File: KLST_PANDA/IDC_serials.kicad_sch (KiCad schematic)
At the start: 0 parts

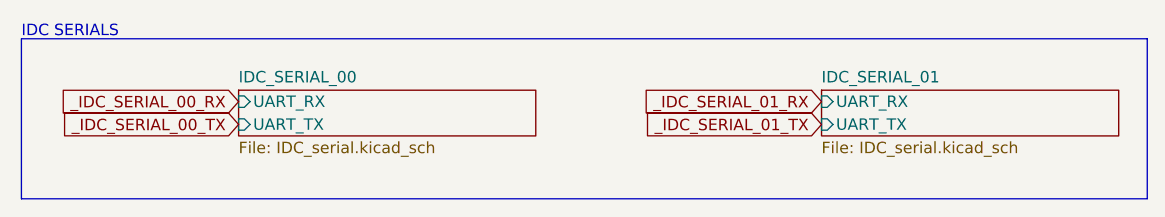
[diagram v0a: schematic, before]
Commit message: continued routing
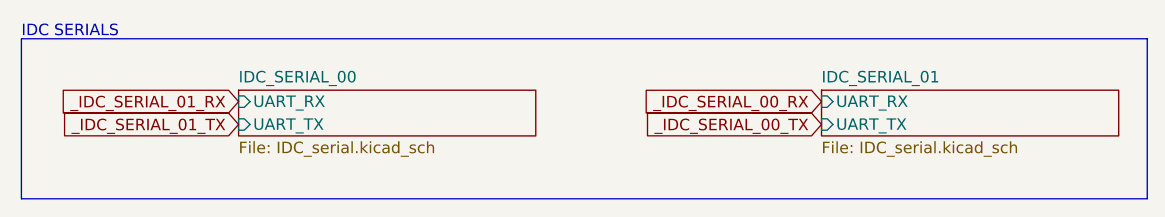
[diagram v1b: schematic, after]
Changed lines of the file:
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@@
     (effects (font (size 1.27 1.27)) (justify left bottom))
   )
-  (global_label "_IDC_SERIAL_00_TX" (shape input) (at 39.37 24.765 180) (fields_autoplaced)
+  (global_label "_IDC_SERIAL_00_TX" (shape input) (at 104.14 24.765 180) (fields_autoplaced)
+    (effects (font (size 1.27 1.27)) (justify right))
+    (property "Intersheetrefs" "${INTERSHEET_REFS}" (at 83.2729 24.765 0)
+      (effects (font (size 1.27 1.27)) (justify right) hide)
+    )
+  )
+  (global_label "_IDC_SERIAL_01_TX" (shape input) (at 39.37 24.765 180) (fields_autoplaced)
     (effects (font (size 1.27 1.27)) (justify right))
     (property "Intersheetrefs" "${INTERSHEET_REFS}" (at 18.5029 24.765 0)
@@
     )
   )
-  (global_label "_IDC_SERIAL_01_TX" (shape input) (at 104.14 24.765 180) (fields_autoplaced)
+  (global_label "_IDC_SERIAL_00_RX" (shape input) (at 104.14 22.225 180) (fields_autoplaced)
     (effects (font (size 1.27 1.27)) (justify right))
-    (property "Intersheetrefs" "${INTERSHEET_REFS}" (at 83.2729 24.765 0)
+    (property "Intersheetrefs" "${INTERSHEET_REFS}" (at 82.9705 22.225 0)
       (effects (font (size 1.27 1.27)) (justify right) hide)
     )
   )
-  (global_label "_IDC_SERIAL_00_RX" (shape input) (at 39.37 22.225 180) (fields_autoplaced)
+  (global_label "_IDC_SERIAL_01_RX" (shape input) (at 39.37 22.225 180) (fields_autoplaced)
     (effects (font (size 1.27 1.27)) (justify right))
     (property "Intersheetrefs" "${INTERSHEET_REFS}" (at 18.2005 22.225 0)
       (effects (font (size 1.27 1.27)) (justify right) hide)
     )
-  )
-  (global_label "_IDC_SERIAL_01_RX" (shape input) (at 104.14 22.225 180) (fields_autoplaced)
-    (effects (font (size 1.27 1.27)) (justify right))
-    (property "Intersheetrefs" "${INTERSHEET_REFS}" (at 82.9705 22.225 0)
-      (effects (font (size 1.27 1.27)) (justify right) hide)
-    )
